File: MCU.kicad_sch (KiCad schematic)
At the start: 29 parts, among them J3 Conn_01x02_Socket, J4 Conn_01x02_Socket, U3 TPS56A37RPAR, U4 ATSAMD21G18A-A

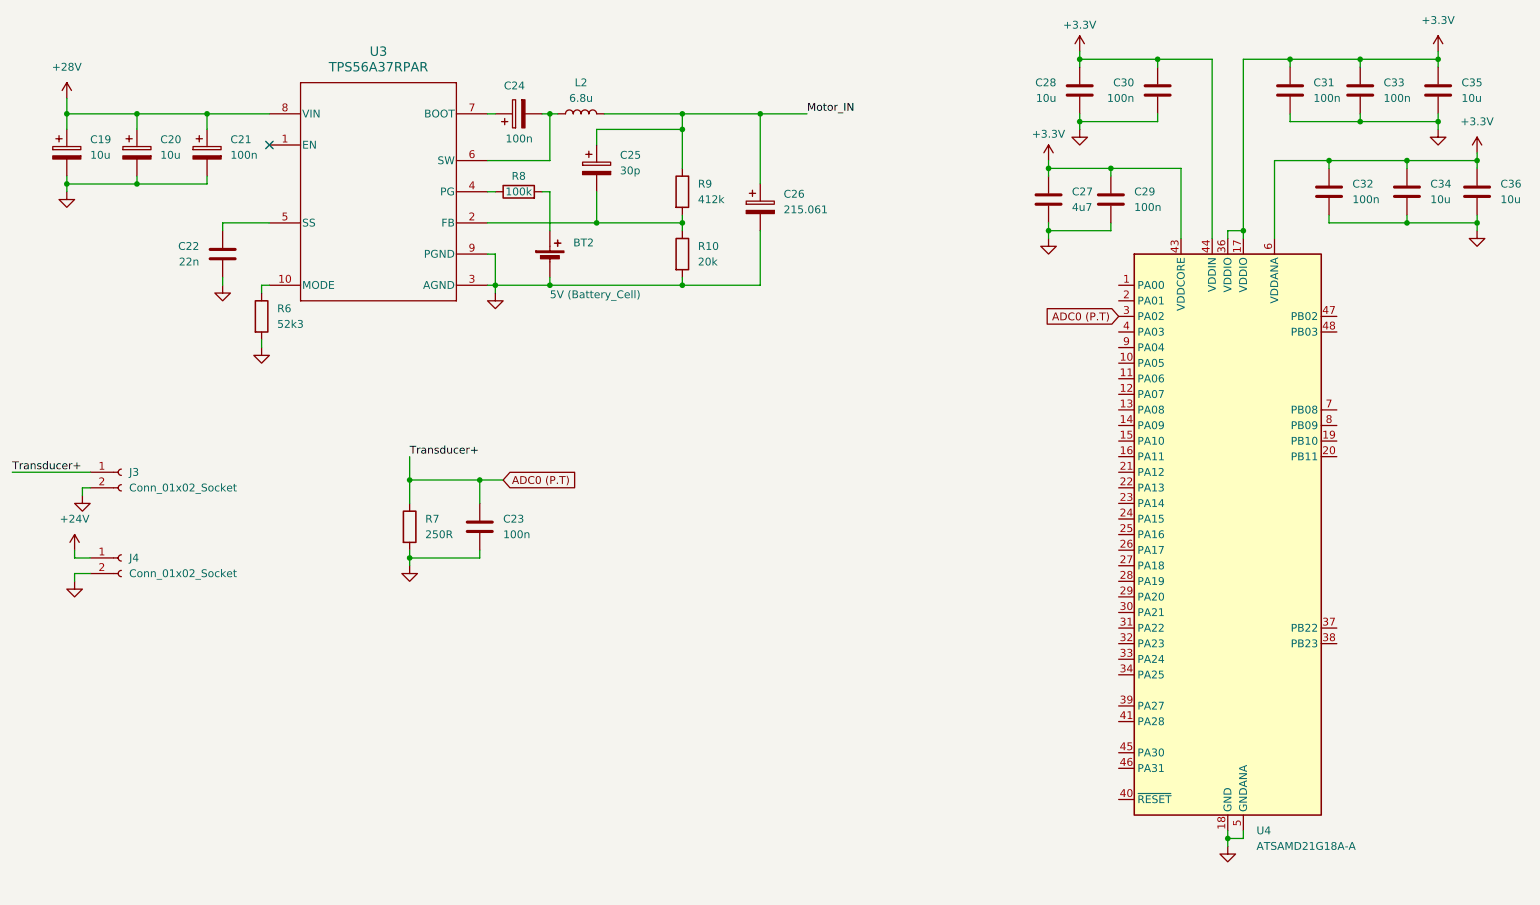
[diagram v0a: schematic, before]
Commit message: Added USB C, LDO regulator and sections off schematic in pages to make readable
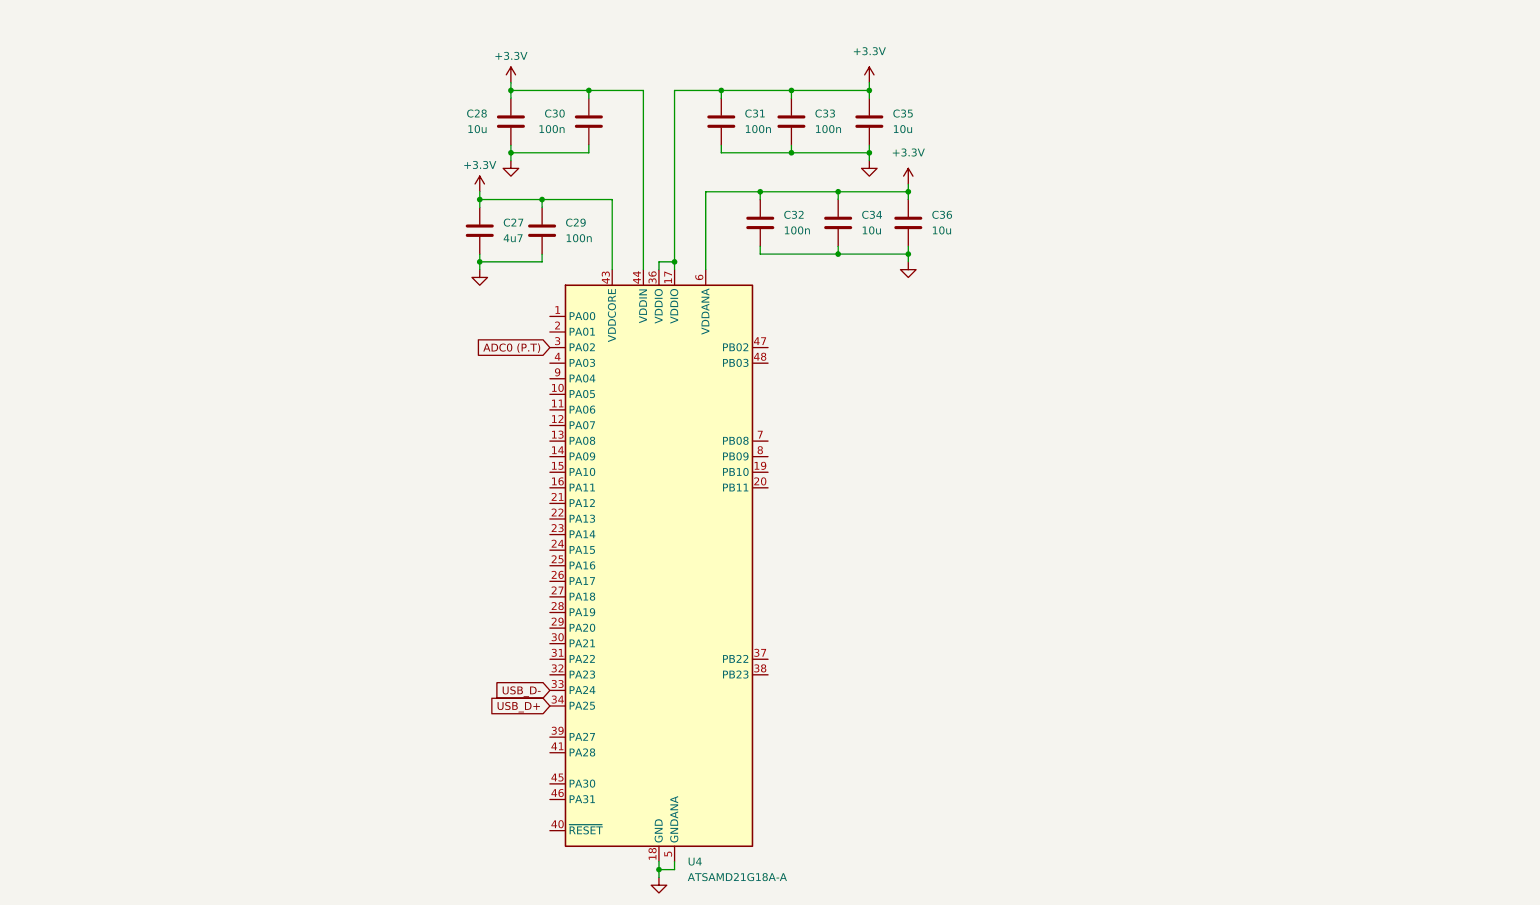
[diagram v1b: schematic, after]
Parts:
- removed BT2: 5V (Battery_Cell), symbol Device:Battery_Cell
- removed C19, C20: 10u, symbol Device:C_Polarized
- removed C21, C24: 100n, symbol Device:C_Polarized
- removed C22: 22n, symbol Device:C
- removed C23: 100n, symbol Device:C
- removed C25: 30p, symbol Device:C_Polarized
- removed C26: 215.061, symbol Device:C_Polarized
- removed J3, J4: Conn_01x02_Socket, symbol Connector:Conn_01x02_Socket
- removed L2: 6.8u, symbol Device:L
- removed R10: 20k, symbol Device:R
- removed R6: 52k3, symbol Device:R
- removed R7: 250R, symbol Device:R
- removed R8: 100k, symbol Device:R
- removed R9: 412k, symbol Device:R
- removed U3: TPS56A37RPAR, RPA0010A-MFG, symbol Imported_ICs:TPS56A37RPAR
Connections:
- net USB_D-: now reaches U4.33 (PA24)
- net USB_D+: now reaches U4.34 (PA25)
- no-connect marks 1 -> 0
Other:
- moved on the sheet: C27, C28, C29, C30, C31, C32, C33, C34, C35, C36, U4
